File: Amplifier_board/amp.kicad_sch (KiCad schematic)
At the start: 43 parts, among them J11 Conn_01x03_Pin, J15 Conn_01x03_Pin, U4 TPA3111D1PWPR

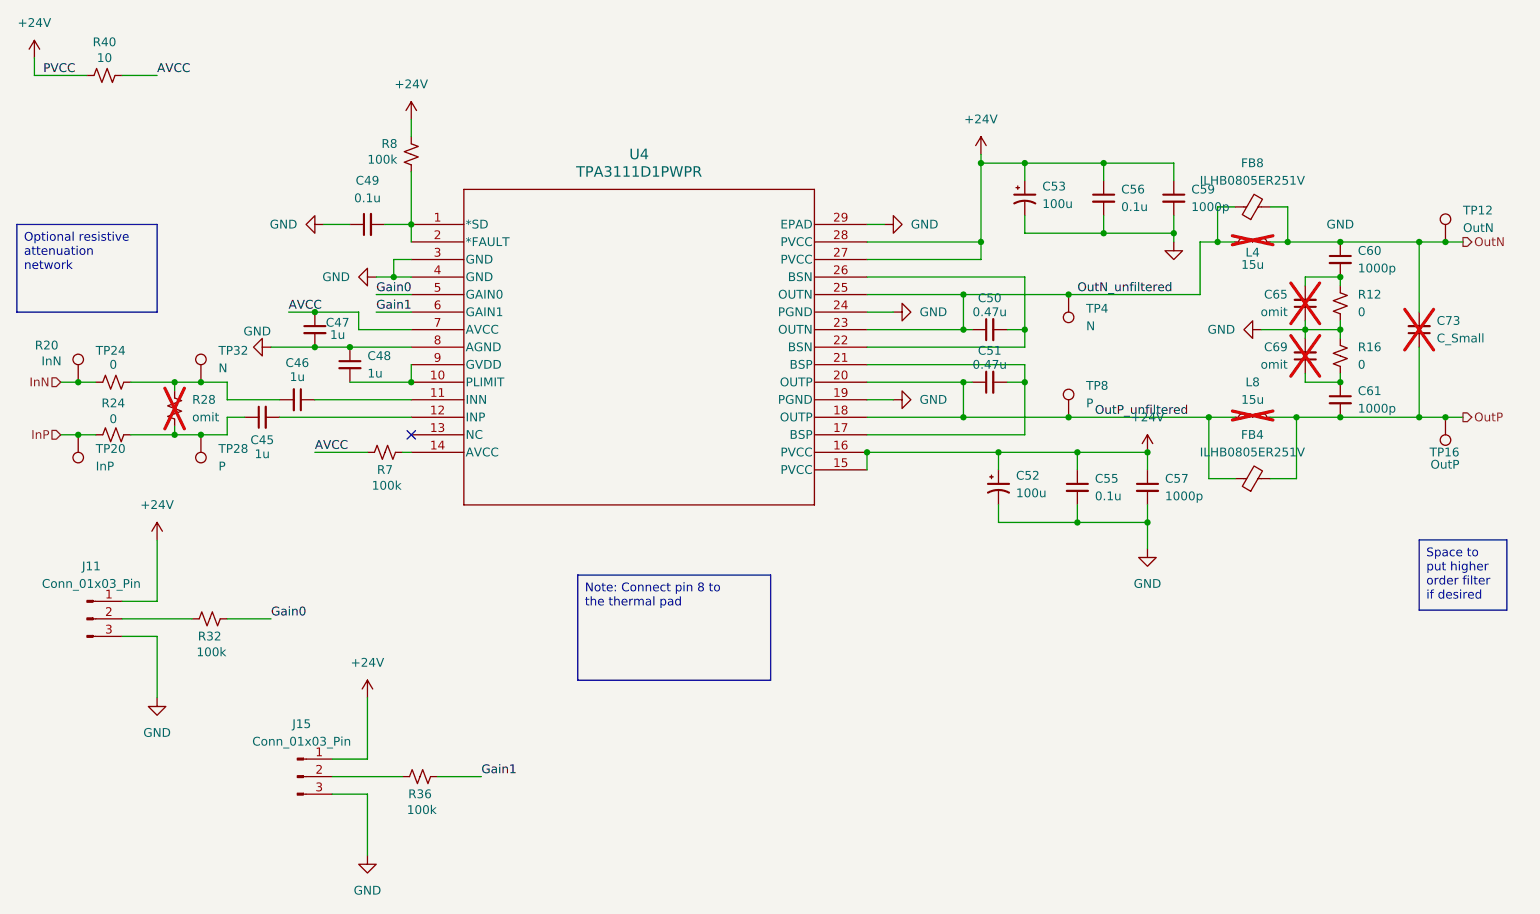
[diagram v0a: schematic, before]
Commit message: generated gerber files
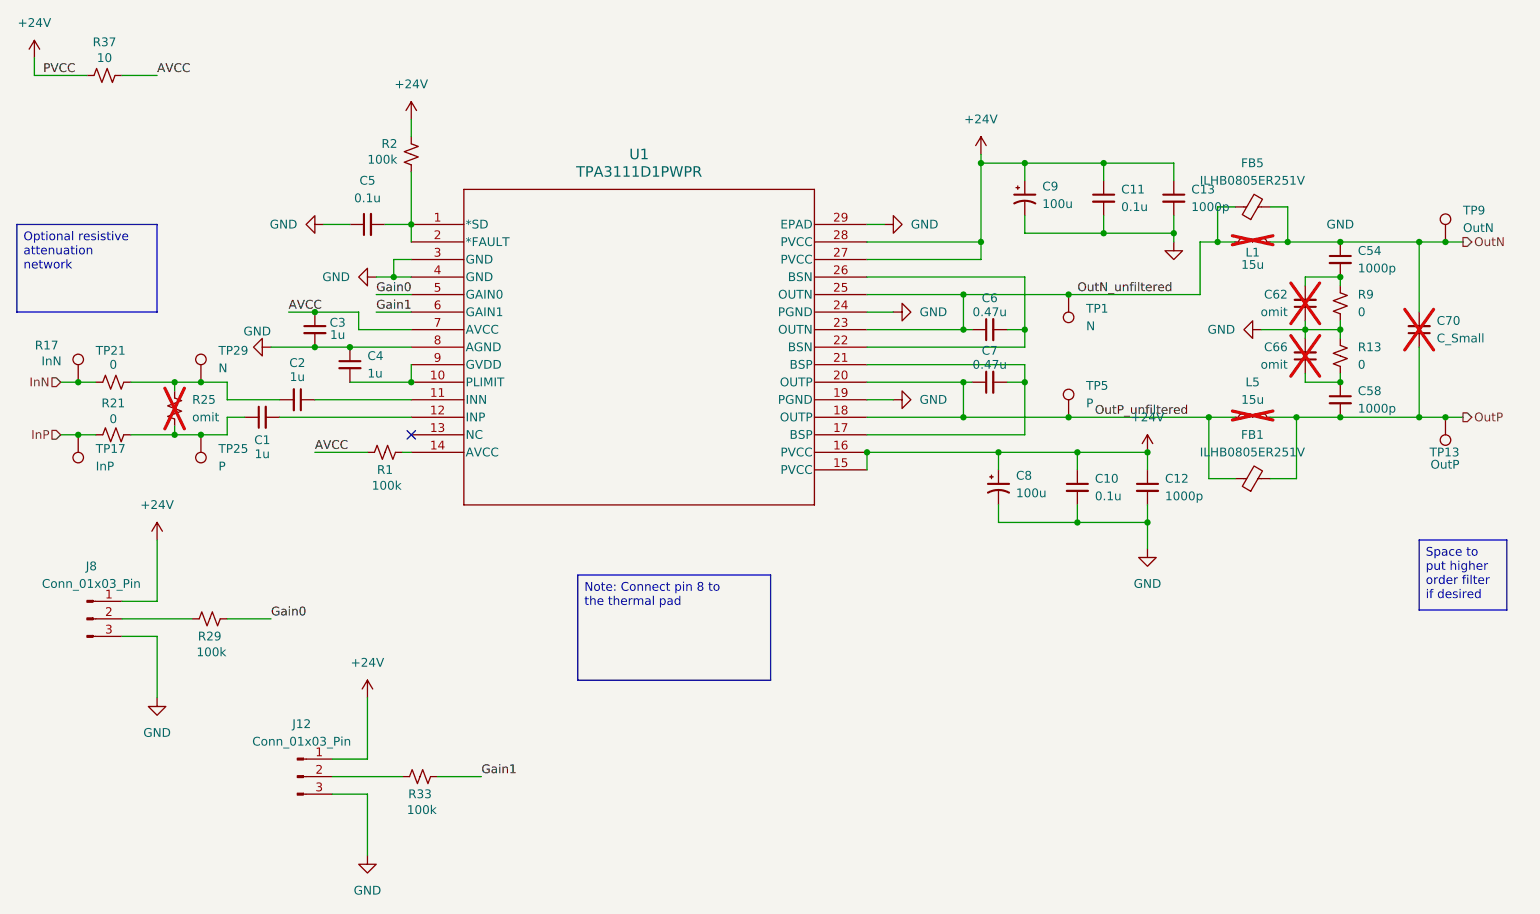
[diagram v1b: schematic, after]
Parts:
- renumbered C45 to C1, C55 to C10, C56 to C11, C57 to C12, C59 to C13, C46 to C2, C47 to C3, C48 to C4, C49 to C5, C60 to C54, C61 to C58, C50 to C6, C65 to C62, C69 to C66, C51 to C7, C73 to C70, C52 to C8, C53 to C9, FB4 to FB1, FB8 to FB5, J15 to J12, J11 to J8, L4 to L1, L8 to L5, R7 to R1, R16 to R13, R20 to R17, R8 to R2, R24 to R21, R28 to R25, R32 to R29, R36 to R33, R40 to R37, R12 to R9, TP4 to TP1, TP16 to TP13, TP20 to TP17, TP24 to TP21, TP28 to TP25, TP32 to TP29, TP8 to TP5, TP12 to TP9, U4 to U1
